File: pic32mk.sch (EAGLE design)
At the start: 35 parts, among them IC1 PIC32MK1024MCF100-I_PT, IC2 ADM3095EBRZ, IC3 PIC32MK1024MCF100-I_PT, IC4 MAX203ECWP

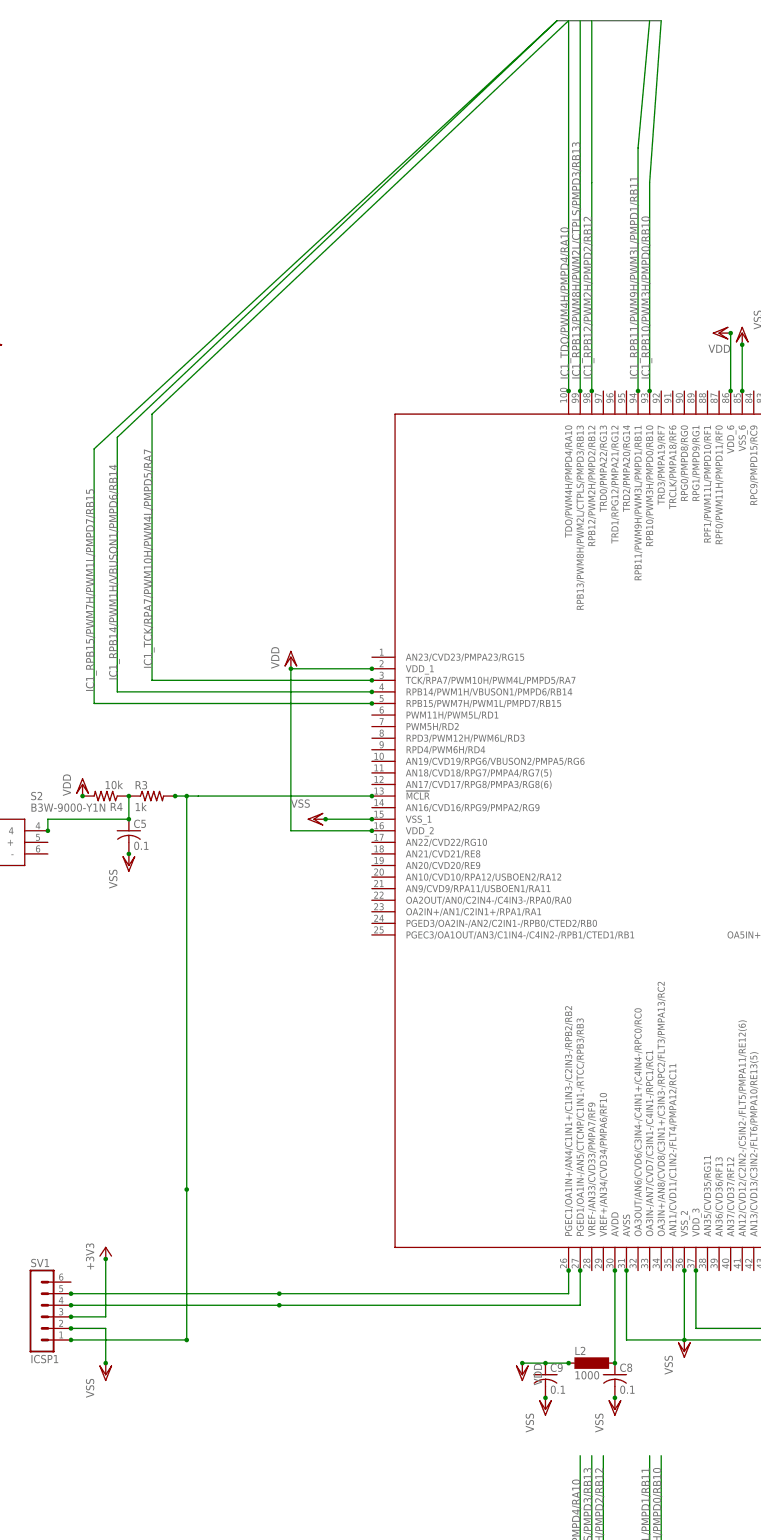
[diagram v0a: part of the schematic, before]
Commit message: up
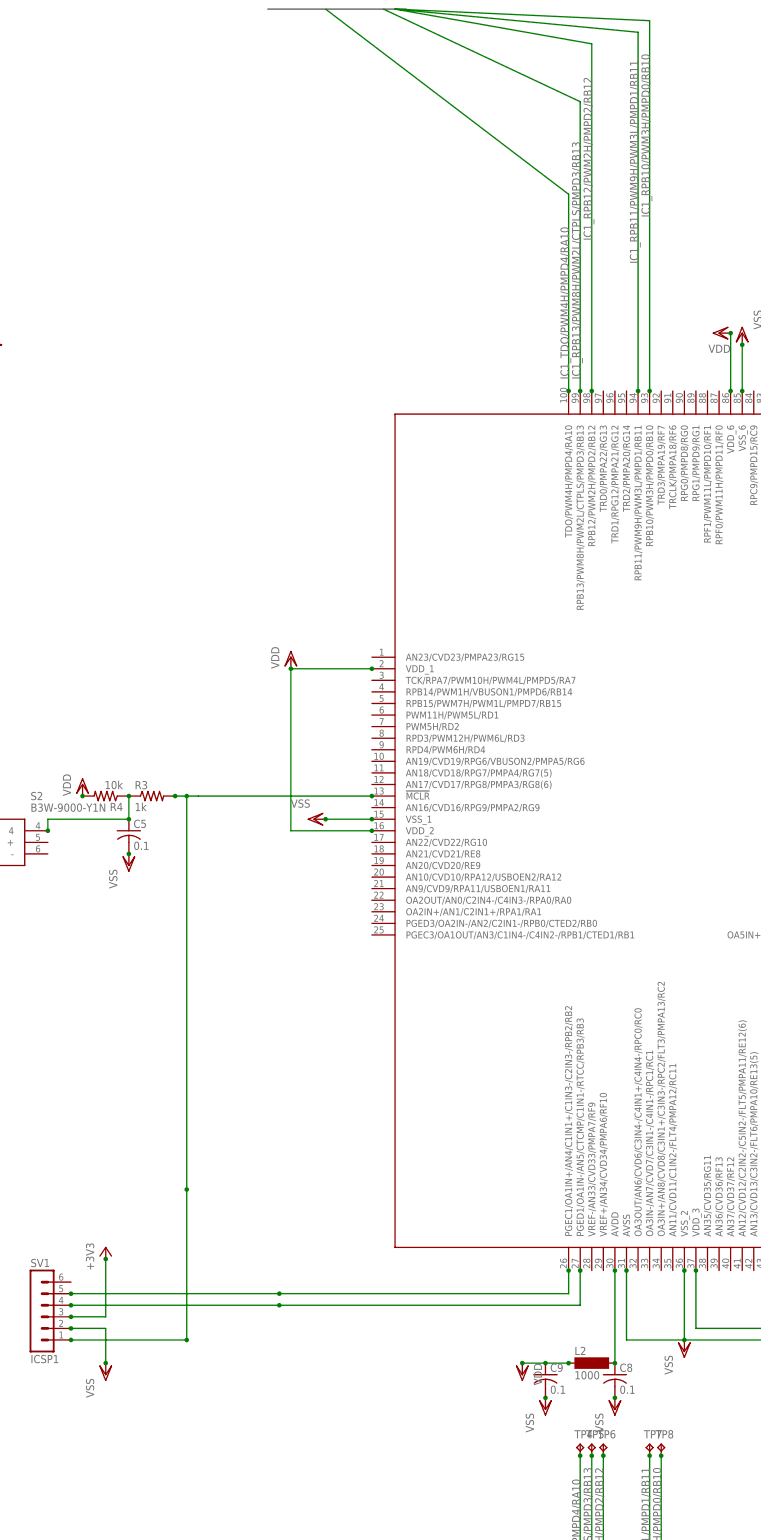
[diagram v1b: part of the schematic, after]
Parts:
- added TP4, TP5, TP6, TP7, TP8: TPB1,27, testpad:TPB1,27
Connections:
- net IC1_RPB10/PWM3H/PMPD0/RB10: now also TP8.TP
- net IC1_RPB11/PWM9H/PWM3L/PMPD1/RB11: now also TP7.TP
- net IC1_RPB12/PWM2H/PMPD2/RB12: now also TP6.TP
- net IC1_RPB13/PWM8H/PWM2L/CTPLS/PMPD3/RB13: now also TP5.TP
- net IC1_RPB14/PWM1H/VBUSON1/PMPD6/RB14: no longer IC3.RPB14/PWM1H/VBUSON1/PMPD6/RB14
- net IC1_RPB15/PWM7H/PWM1L/PMPD7/RB15: no longer IC3.RPB15/PWM7H/PWM1L/PMPD7/RB15
- net IC1_TCK/RPA7/PWM10H/PWM4L/PMPD5/RA7: no longer IC3.TCK/RPA7/PWM10H/PWM4L/PMPD5/RA7
- net IC1_TDO/PWM4H/PMPD4/RA10: now also TP4.TP
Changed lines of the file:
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@@
 <part name="VDD18" library="supply1" library_urn="urn:adsk.eagle:library:371" deviceset="VDD" device=""/>
 <part name="VSS29" library="supply1" library_urn="urn:adsk.eagle:library:371" deviceset="VSS" device=""/>
+<part name="TP4" library="testpad" library_urn="urn:adsk.eagle:library:385" deviceset="TP" device="B1,27" package3d_urn="urn:adsk.eagle:package:27944/2"/>
+<part name="TP5" library="testpad" library_urn="urn:adsk.eagle:library:385" deviceset="TP" device="B1,27" package3d_urn="urn:adsk.eagle:package:27944/2"/>
+<part name="TP6" library="testpad" library_urn="urn:adsk.eagle:library:385" deviceset="TP" device="B1,27" package3d_urn="urn:adsk.eagle:package:27944/2"/>
+<part name="TP7" library="testpad" library_urn="urn:adsk.eagle:library:385" deviceset="TP" device="B1,27" package3d_urn="urn:adsk.eagle:package:27944/2"/>
+<part name="TP8" library="testpad" library_urn="urn:adsk.eagle:library:385" deviceset="TP" device="B1,27" package3d_urn="urn:adsk.eagle:package:27944/2"/>
 </parts>
 <sheets>
@@
 <attribute name="VALUE" x="254" y="58.42" size="1.778" layer="96" rot="R270"/>
 </instance>
+<instance part="TP4" gate="G$1" x="55.88" y="170.18" smashed="yes">
+<attribute name="NAME" x="54.61" y="171.45" size="1.778" layer="95"/>
+<attribute name="TP_SIGNAL_NAME" x="57.15" y="168.91" size="1.778" layer="97"/>
+</instance>
+<instance part="TP5" gate="G$1" x="58.42" y="170.18" smashed="yes">
+<attribute name="NAME" x="57.15" y="171.45" size="1.778" layer="95"/>
+<attribute name="TP_SIGNAL_NAME" x="59.69" y="168.91" size="1.778" layer="97"/>
+</instance>
+<instance part="TP6" gate="G$1" x="60.96" y="170.18" smashed="yes">
+<attribute name="NAME" x="59.69" y="171.45" size="1.778" layer="95"/>
+<attribute name="TP_SIGNAL_NAME" x="62.23" y="168.91" size="1.778" layer="97"/>
+</instance>
+<instance part="TP7" gate="G$1" x="71.12" y="170.18" smashed="yes">
+<attribute name="NAME" x="69.85" y="171.45" size="1.778" layer="95"/>
+<attribute name="TP_SIGNAL_NAME" x="72.39" y="168.91" size="1.778" layer="97"/>
+</instance>
+<instance part="TP8" gate="G$1" x="73.66" y="170.18" smashed="yes">
+<attribute name="NAME" x="72.39" y="171.45" size="1.778" layer="95"/>
+<attribute name="TP_SIGNAL_NAME" x="74.93" y="168.91" size="1.778" layer="97"/>
+</instance>
 </instances>
 <busses>
 <bus name="DPMP1:IC1_RPB10/PWM3H/PMPD0/RB10,IC1_RPB11/PWM9H/PWM3L/PMPD1/RB11,IC1_RPB12/PWM2H/PMPD2/RB12,IC1_RPB13/PWM8H/PWM2L/CTPLS/PMPD3/RB13,IC1_RPB14/PWM1H/VBUSON1/PMPD6/RB14,IC1_RPB15/PWM7H/PWM1L/PMPD7/RB15,IC1_TCK/RPA7/PWM10H/PWM4L/PMPD5/RA7,IC1_TDO/PWM4H/PMPD4/RA10">
 <segment>
-<wire x1="50.8" y1="482.6" x2="73.66" y2="482.6" width="0.762" layer="92"/>
+<wire x1="-12.7" y1="485.14" x2="17.78" y2="485.14" width="0.762" layer="92"/>
 </segment>
 </bus>
@@
 <junction x="12.7" y="40.64"/>
 </segment>
-<segment>
-<wire x1="53.34" y1="482.6" x2="-38.1" y2="396.24" width="0.1524" layer="91"/>
-<wire x1="-38.1" y1="396.24" x2="-38.1" y2="337.82" width="0.1524" layer="91"/>
-<label x="-38.1" y="340.36" size="1.778" layer="95" rot="R90"/>
-<pinref part="IC3" gate="G$1" pin="TCK/RPA7/PWM10H/PWM4L/PMPD5/RA7"/>
-<wire x1="10.16" y1="337.82" x2="-38.1" y2="337.82" width="0.1524" layer="91"/>
-<junction x="10.16" y="337.82"/>
-</segment>
 </net>
 <net name="IC1_RPB14/PWM1H/VBUSON1/PMPD6/RB14" class="0">
@@
 <junction x="12.7" y="38.1"/>
 </segment>
-<segment>
-<wire x1="50.8" y1="482.6" x2="-45.72" y2="391.16" width="0.1524" layer="91"/>
-<wire x1="-45.72" y1="391.16" x2="-45.72" y2="335.28" width="0.1524" layer="91"/>
-<label x="-45.72" y="337.82" size="1.778" layer="95" rot="R90"/>
-<pinref part="IC3" gate="G$1" pin="RPB14/PWM1H/VBUSON1/PMPD6/RB14"/>
-<wire x1="10.16" y1="335.28" x2="-45.72" y2="335.28" width="0.1524" layer="91"/>
-<junction x="10.16" y="335.28"/>
-</segment>
 </net>
 <net name="IC1_RPB15/PWM7H/PWM1L/PMPD7/RB15" class="0">
@@
 <junction x="12.7" y="35.56"/>
 </segment>
-<segment>
-<wire x1="50.8" y1="482.6" x2="-50.8" y2="388.62" width="0.1524" layer="91"/>
-<wire x1="-50.8" y1="388.62" x2="-50.8" y2="332.74" width="0.1524" layer="91"/>
-<label x="-50.8" y="335.28" size="1.778" layer="95" rot="R90"/>
-<pinref part="IC3" gate="G$1" pin="RPB15/PWM7H/PWM1L/PMPD7/RB15"/>
-<wire x1="10.16" y1="332.74" x2="-50.8" y2="332.74" width="0.1524" layer="91"/>
-<junction x="10.16" y="332.74"/>
-</segment>
 </net>
 <net name="IC1_TDO/PWM4H/PMPD4/RA10" class="0">
@@
 <label x="55.88" y="162.56" size="1.778" layer="95" rot="R90" align="bottom-right"/>
 <junction x="55.88" y="104.14"/>
-</segment>
-<segment>
-<wire x1="53.34" y1="482.6" x2="53.34" y2="401.32" width="0.1524" layer="91"/>
+<junction x="55.88" y="167.64"/>
+<pinref part="TP4" gate="G$1" pin="TP"/>
+</segment>
+<segment>
+<wire x1="0" y1="485.14" x2="53.34" y2="444.5" width="0.1524" layer="91"/>
+<wire x1="53.34" y1="444.5" x2="53.34" y2="401.32" width="0.1524" layer="91"/>
 <label x="53.34" y="403.86" size="1.778" layer="95" rot="R90"/>
 <pinref part="IC3" gate="G$1" pin="TDO/PWM4H/PMPD4/RA10"/>
@@
 <label x="58.42" y="165.1" size="1.778" layer="95" rot="R90" align="bottom-right"/>
 <junction x="58.42" y="104.14"/>
-</segment>
-<segment>
-<wire x1="55.88" y1="482.6" x2="55.88" y2="401.32" width="0.1524" layer="91"/>
+<junction x="58.42" y="167.64"/>
+<pinref part="TP5" gate="G$1" pin="TP"/>
+</segment>
+<segment>
+<wire x1="12.7" y1="485.14" x2="55.88" y2="464.82" width="0.1524" layer="91"/>
+<wire x1="55.88" y1="464.82" x2="55.88" y2="401.32" width="0.1524" layer="91"/>
 <label x="55.88" y="403.86" size="1.778" layer="95" rot="R90"/>
 <pinref part="IC3" gate="G$1" pin="RPB13/PWM8H/PWM2L/CTPLS/PMPD3/RB13"/>
@@
 <label x="60.96" y="165.1" size="1.778" layer="95" rot="R90" align="bottom-right"/>
 <junction x="60.96" y="104.14"/>
-</segment>
-<segment>
-<wire x1="58.42" y1="482.6" x2="58.42" y2="447.04" width="0.1524" layer="91"/>
-<wire x1="58.42" y1="447.04" x2="58.42" y2="401.32" width="0.1524" layer="91"/>
-<label x="58.42" y="403.86" size="1.778" layer="95" rot="R90"/>
+<junction x="60.96" y="167.64"/>
+<pinref part="TP6" gate="G$1" pin="TP"/>
+</segment>
+<segment>
+<wire x1="15.24" y1="485.14" x2="58.42" y2="477.52" width="0.1524" layer="91"/>
+<wire x1="58.42" y1="477.52" x2="58.42" y2="401.32" width="0.1524" layer="91"/>
+<label x="58.42" y="434.34" size="1.778" layer="95" rot="R90"/>
 <pinref part="IC3" gate="G$1" pin="RPB12/PWM2H/PMPD2/RB12"/>
 <junction x="58.42" y="401.32"/>
@@
 <label x="71.12" y="165.1" size="1.778" layer="95" rot="R90" align="bottom-right"/>
 <junction x="71.12" y="104.14"/>
-</segment>
-<segment>
-<wire x1="71.12" y1="482.6" x2="68.58" y2="454.66" width="0.1524" layer="91"/>
-<wire x1="68.58" y1="454.66" x2="68.58" y2="401.32" width="0.1524" layer="91"/>
-<label x="68.58" y="403.86" size="1.778" layer="95" rot="R90"/>
+<junction x="71.12" y="167.64"/>
+<pinref part="TP7" gate="G$1" pin="TP"/>
+</segment>
+<segment>
+<wire x1="15.24" y1="485.14" x2="68.58" y2="480.06" width="0.1524" layer="91"/>
+<wire x1="68.58" y1="480.06" x2="68.58" y2="401.32" width="0.1524" layer="91"/>
+<label x="68.58" y="429.26" size="1.778" layer="95" rot="R90"/>
 <pinref part="IC3" gate="G$1" pin="RPB11/PWM9H/PWM3L/PMPD1/RB11"/>
 <junction x="68.58" y="401.32"/>
@@
 <label x="73.66" y="165.1" size="1.778" layer="95" rot="R90" align="bottom-right"/>
 <junction x="73.66" y="104.14"/>
-</segment>
-<segment>
-<wire x1="73.66" y1="482.6" x2="71.12" y2="447.04" width="0.1524" layer="91"/>
-<wire x1="71.12" y1="447.04" x2="71.12" y2="401.32" width="0.1524" layer="91"/>
-<label x="71.12" y="403.86" size="1.778" layer="95" rot="R90"/>
+<junction x="73.66" y="167.64"/>
+<pinref part="TP8" gate="G$1" pin="TP"/>
+</segment>
+<segment>
+<wire x1="15.24" y1="485.14" x2="71.12" y2="482.6" width="0.1524" layer="91"/>
+<wire x1="71.12" y1="482.6" x2="71.12" y2="401.32" width="0.1524" layer="91"/>
+<label x="71.12" y="439.42" size="1.778" layer="95" rot="R90"/>
 <pinref part="IC3" gate="G$1" pin="RPB10/PWM3H/PMPD0/RB10"/>
 <junction x="71.12" y="401.32"/>

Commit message: up
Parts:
- removed TP5, TP6, TP7, TP8: TPB1,27, testpad:TPB1,27
- added TP1, TP2, TP3: TPB1,27, testpad:TPB1,27
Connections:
- removed net IC1_RPB14/PWM1H/VBUSON1/PMPD6/RB14: IC1.RPB14/PWM1H/VBUSON1/PMPD6/RB14
- removed net IC1_RPB15/PWM7H/PWM1L/PMPD7/RB15: IC1.RPB15/PWM7H/PWM1L/PMPD7/RB15
- removed net IC1_TCK/RPA7/PWM10H/PWM4L/PMPD5/RA7: IC1.TCK/RPA7/PWM10H/PWM4L/PMPD5/RA7
- new net N$10: IC1.TCK/RPA7/PWM10H/PWM4L/PMPD5/RA7, IC3.TCK/RPA7/PWM10H/PWM4L/PMPD5/RA7
- new net N$15: IC1.RPB14/PWM1H/VBUSON1/PMPD6/RB14, IC3.RPB14/PWM1H/VBUSON1/PMPD6/RB14
- new net N$17: IC1.RPB15/PWM7H/PWM1L/PMPD7/RB15, IC3.RPB15/PWM7H/PWM1L/PMPD7/RB15
- net IC1_RPB10/PWM3H/PMPD0/RB10: no longer TP8.TP
- net IC1_RPB11/PWM9H/PWM3L/PMPD1/RB11: no longer TP7.TP
- net IC1_RPB12/PWM2H/PMPD2/RB12: no longer TP6.TP
- net IC1_RPB13/PWM8H/PWM2L/CTPLS/PMPD3/RB13: no longer TP5.TP
- net IC1_TDO/PWM4H/PMPD4/RA10: no longer TP4.TP
- net VDD: now also IC1.VDD_5, IC3.VDD_5, TP1.TP, TP2.TP
- net VSS: now also TP3.TP, TP4.TP
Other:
- moved on the sheet: TP4
